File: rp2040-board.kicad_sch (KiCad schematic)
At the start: 101 parts

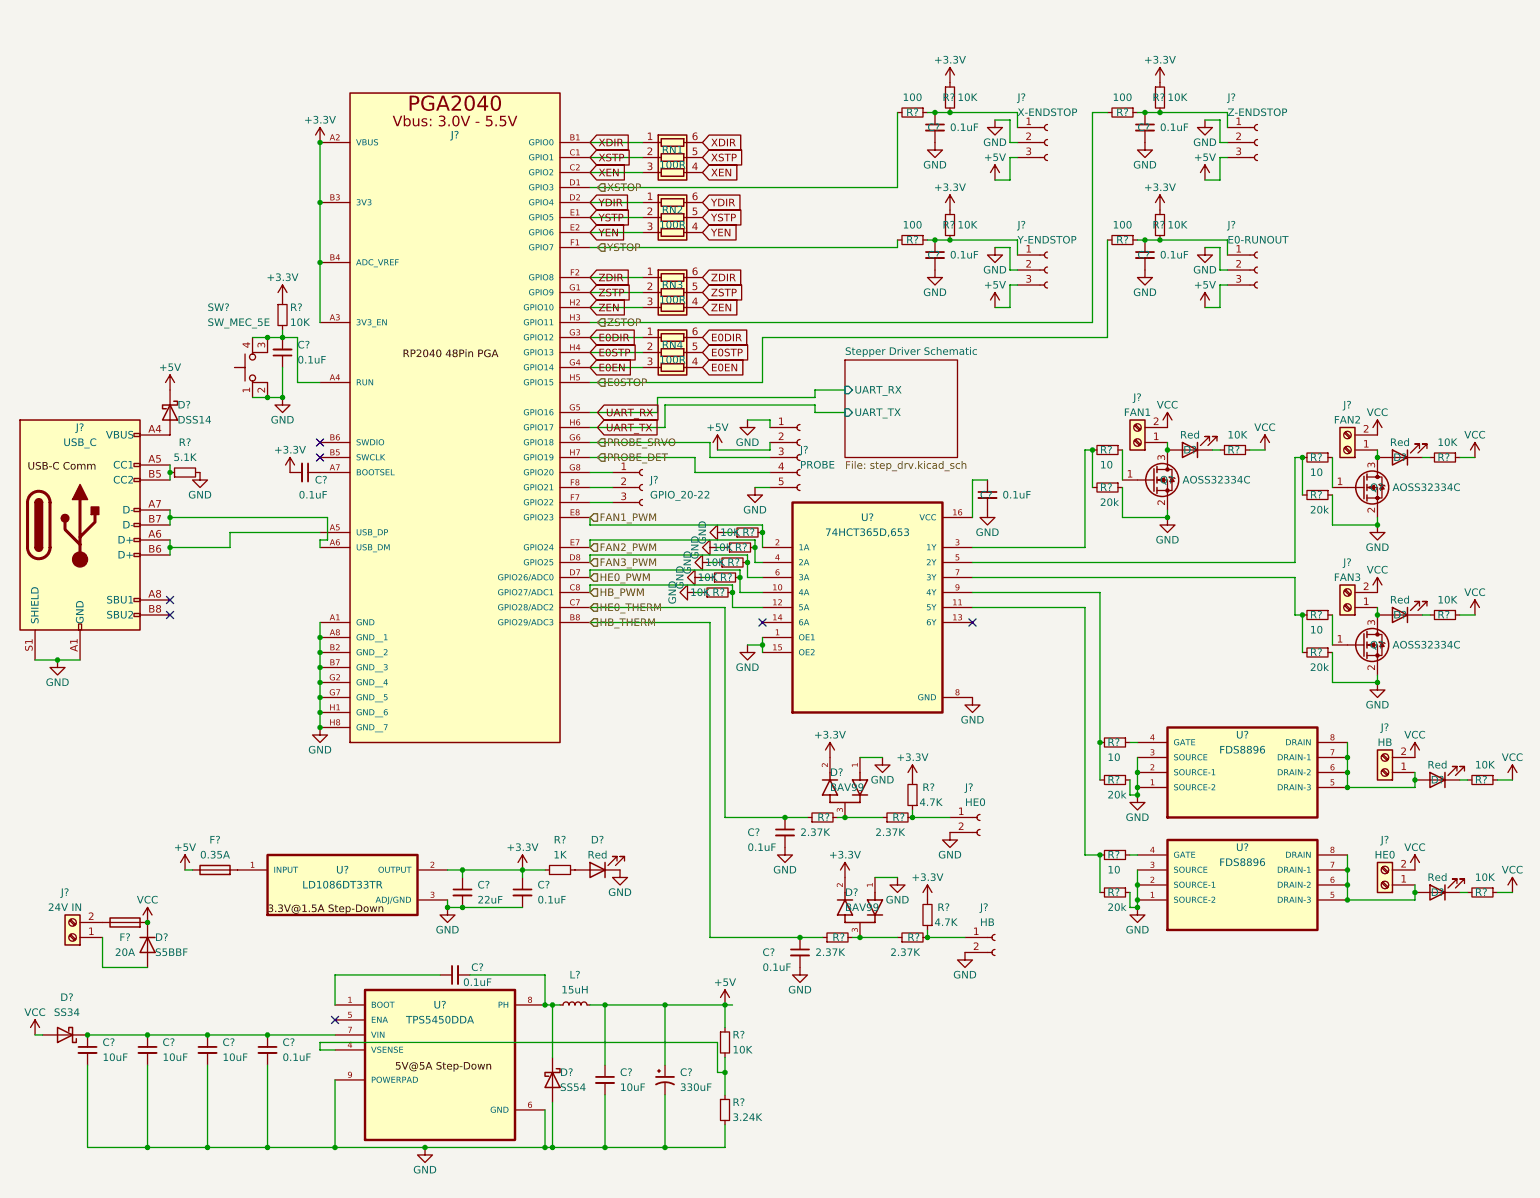
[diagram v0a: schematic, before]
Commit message: Finished Schematic
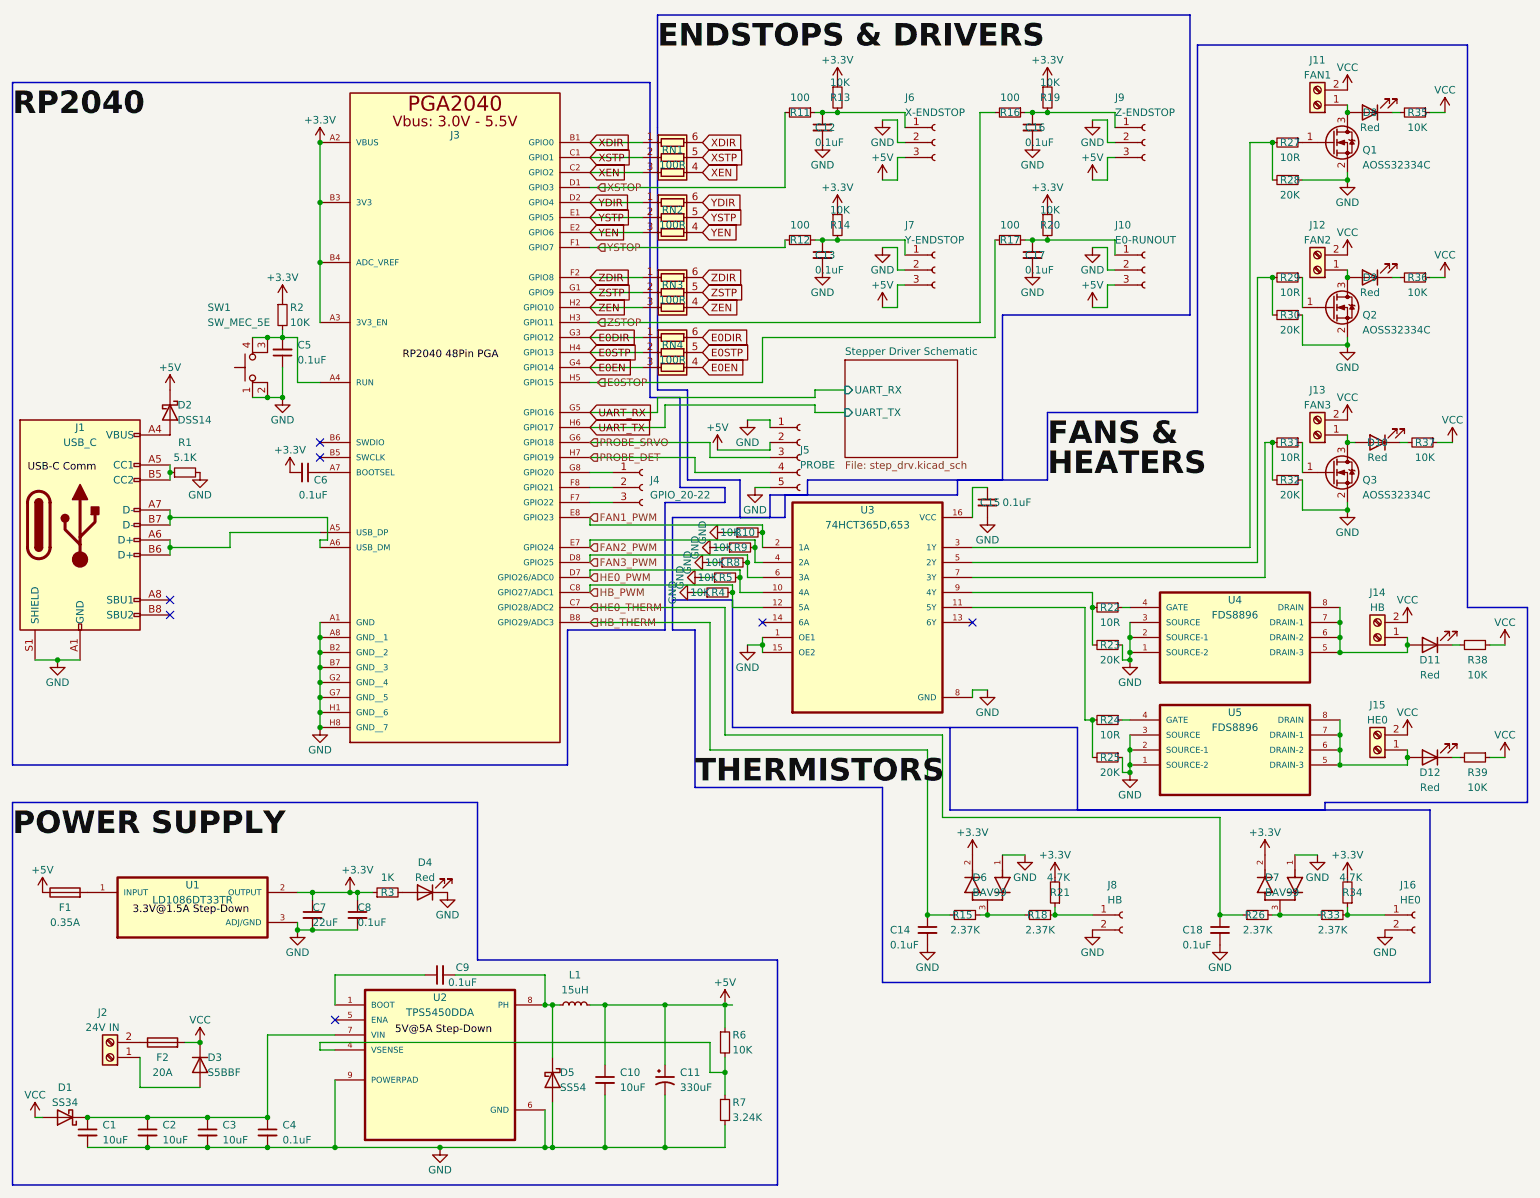
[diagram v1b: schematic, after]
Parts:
- R22, R24, R27, R29, R31: renamed from R?; value 10 -> 10R
- R23, R25, R28, R30, R32: renamed from R?; value 20k -> 20K
- gave numbers to parts that had none: 87
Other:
- moved on the sheet: C1, C12, C13, C14, C15, C16, C17, C18, C2, C3, C4, C7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
